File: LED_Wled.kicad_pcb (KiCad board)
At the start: 2 copper layers, 62 x 43 mm, 54 parts, among them J1 SWD_PORT_SKEDD, J2 Barrel_Jack, J3 VIN-Out, J4 MIC_input, J5 LED_signal_chan, J6 +5V Out, Q1 AO4485, Q2 AO4485, Q3 MMBT3904, Q4 AO4485, Q5 AO4485, Q6 MMBT3904, U1 ESP32-WROOM-32, U2 TPS5450DDAR, U3 AMS1117-3.3, U4 SN74HC125DR

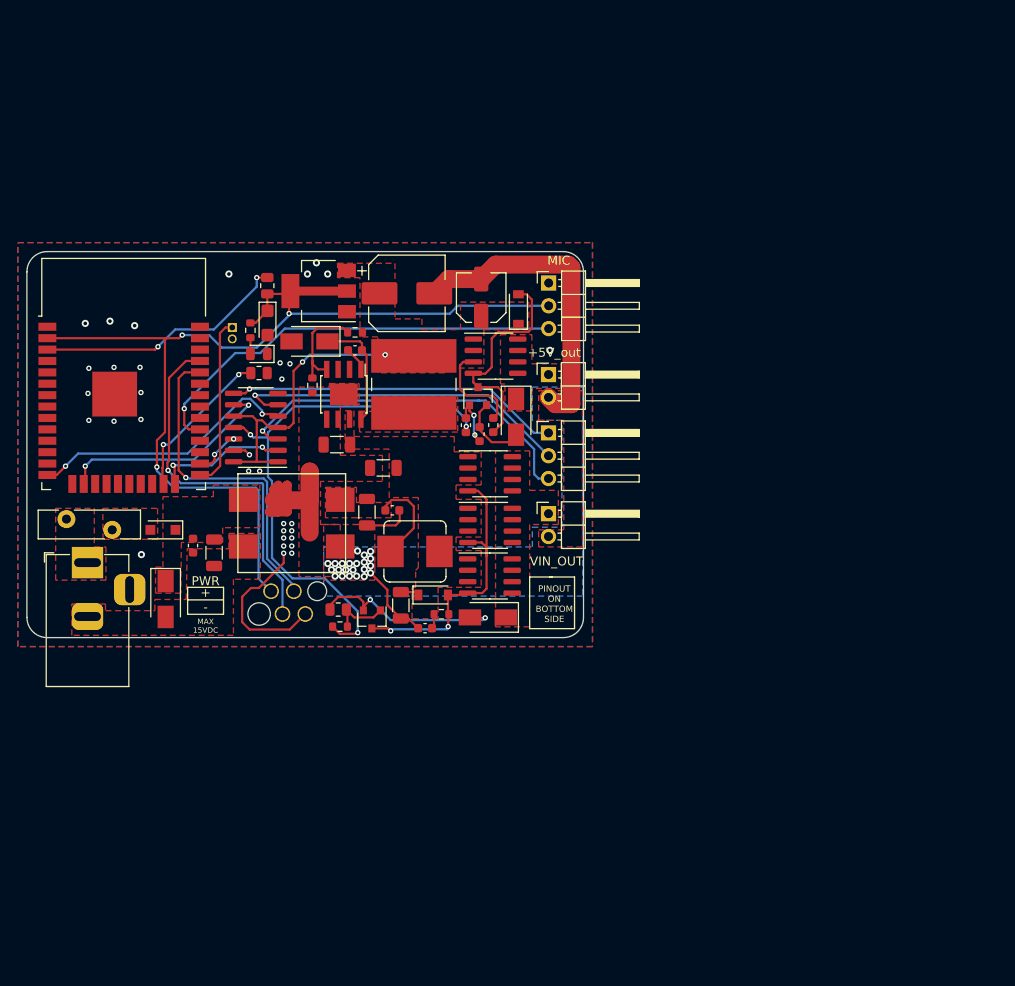
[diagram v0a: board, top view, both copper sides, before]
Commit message: rev2.01
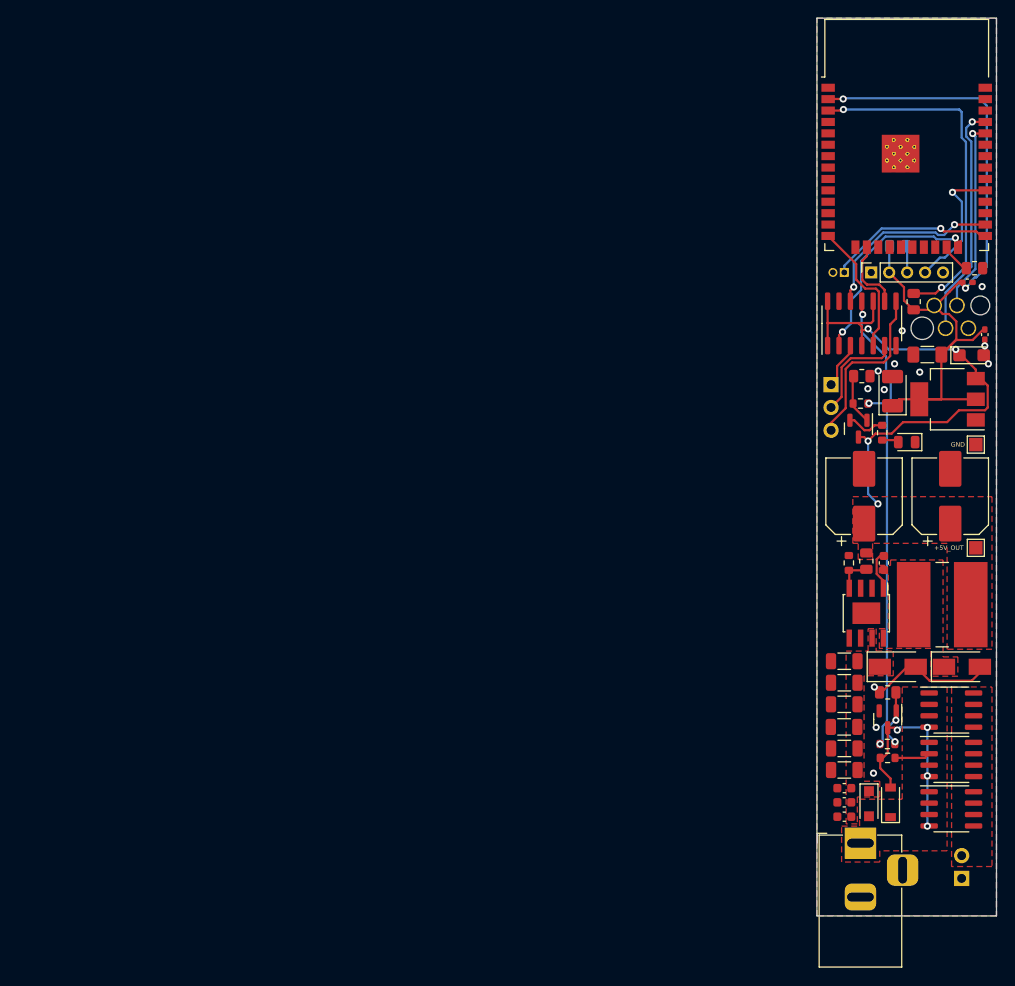
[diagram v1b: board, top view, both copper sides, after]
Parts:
- removed D6, D8: SS34, Diode_SMD:D_SMA
- removed D7: BZT52B15, Diode_SMD:D_SOD-123
- removed F1: Polyfuse, Fuse:Fuse_Bourns_MF-RG650
- removed the G*** at (139.8, 98.5)
- removed L2: 3.3 µH, 6.6 A, Inductor_SMD:L_Bourns_SRP7028A_7.3x6.6mm
- removed L3: ACM1211, userdvc:ACM1211
- removed NT1: Net-Tie_2, NetTie:NetTie-2_SMD_Pad2.0mm
- removed Q6: MMBT3904, Package_TO_SOT_SMD:SOT-23
- added C13: 220 uF 16V, Capacitor_SMD:CP_Elec_8x6.7, F.Cu at (204.8, 103.2)
- added C14: 10uF 16V, Capacitor_Tantalum_SMD:CP_EIA-3216-10_Kemet-I, F.Cu at (207.2, 87.5)
- added C15: 100nF 16V, Capacitor_SMD:C_0402_1005Metric_Pad0.74x0.62mm_HandSolder, F.Cu at (208.7, 85.2)
- added C16: 1uF 25V, Capacitor_SMD:C_0402_1005Metric_Pad0.74x0.62mm_HandSolder, F.Cu at (206.8, 79.4)
- added C17: 100uF 6.3V, Capacitor_SMD:C_1206_3216Metric_Pad1.33x1.80mm_HandSolder, F.Cu at (202.3, 87.5)
- added G***: LOGO, LED_Wled:easyled, B.Cu at (200.0, 60.0)
- added J7: 5V_TP, TestPoint:TestPoint_Pad_1.5x1.5mm, F.Cu at (207.7, 97.5)
- C2: value 150 uF 16V -> 220 uF 16V
- C3: value 22uF 16V -> 22uF/25V; footprint Capacitor_SMD:C_Elec_5x5.4 -> Capacitor_SMD:C_1206_3216Metric
- C4, C5: value 10uF 50V -> 22uF/25V
- C6: value 22uF 10V -> 100uF 6.3V; footprint Capacitor_Tantalum_SMD:CP_EIA-3216-10_Kemet-I -> Capacitor_Tantalum_SMD:CP_EIA-3528-12_Kemet-T_Pad1.50x2.35mm_HandSolder
- J3: value VIN-Out -> LED_VOut; moved to B.Cu
- J4: value MIC_input -> Microphone connector; footprint Connector_PinHeader_2.54mm:PinHeader_1x03_P2.54mm_Horizontal -> Connector_PinSocket_2.00mm:PinSocket_1x05_P2.00mm_Vertical
- J5: moved to B.Cu
- J6: value +5V Out -> Conn_01x01; footprint Connector_PinHeader_2.54mm:PinHeader_1x02_P2.54mm_Horizontal -> TestPoint:TestPoint_Pad_1.5x1.5mm
- L1: value 22uH/5A -> 10uH/6.5A
- Q1: value AO4485 -> MMBT3904; footprint Package_SO:SOIC-8_3.9x4.9mm_P1.27mm -> Package_TO_SOT_SMD:SOT-23
- R11: footprint Resistor_SMD:R_0603_1608Metric -> Resistor_SMD:R_0805_2012Metric
- R2: value 4.7k -> 47ohm
- R4: value 4.7k -> 10k; footprint Resistor_SMD:R_0603_1608Metric -> Resistor_SMD:R_0805_2012Metric
- R8: value 15k -> 0ohm; footprint Resistor_SMD:R_0603_1608Metric -> Resistor_SMD:R_0805_2012Metric; moved to B.Cu
- R9: value 4.7k -> 3.3k
- moved J2 91.6 mm to (194.8, 141.9)
- moved U1 91.2 mm to (200.0, 66.0)
- moved D3 84.4 mm to (195.8, 137.5), turned to -90 degrees
- moved D4 81.9 mm to (199.0, 122.2), turned to 0 degrees
- moved D2 81.2 mm to (206.2, 122.2), turned to 0 degrees
- moved R3 80.5 mm to (207.6, 77.8)
- moved J1 80.4 mm to (205.0, 83.3)
- moved C7 77.4 mm to (193.1, 135.8), turned to 0 degrees
- moved C8 74.3 mm to (193.1, 133.8), turned to 0 degrees
- moved D1 72.8 mm to (200.0, 97.2)
- moved R1 72.0 mm to (200.8, 81.6)
- moved R2 71.3 mm to (197.3, 96.2)
- moved U3 71.1 mm to (204.6, 92.5)
- moved C6 70.0 mm to (198.4, 91.5), turned to 90 degrees
- moved U4 68.5 mm to (195.0, 84.0), turned to 90 degrees
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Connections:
- net Net-(C1-Pad1) renamed /PH
- net Net-(C1-Pad2) renamed /BOOT
- C10 pad 1: GNDPWR -> GND
- C10 pad 2: Net-(C10-Pad2) -> VIN_F+
- C11 pad 1: GNDPWR -> GND
- C11 pad 2: Vin -> VIN_F+
- C12 pad 1: GNDPWR -> GND
- C12 pad 2: Vin -> VIN_F+
- C2 pad 2: GNDPWR -> GND
- C3 pad 1: +5V -> GND
- C3 pad 2: GNDPWR -> VIN_F+
- C4 pad 1: GNDPWR -> GND
- C4 pad 2: Vin -> VIN_F+
- C5 pad 1: GNDPWR -> GND
- C5 pad 2: Vin -> VIN_F+
- C7 pad 1: VBat- -> GND
- C7 pad 2: /PWR_Line -> VIN_F+
- C8 pad 1: VBat- -> GND
- C8 pad 2: /PWR_Line -> VIN_F+
- C9 pad 1: GNDPWR -> GND
- C9 pad 2: Net-(C10-Pad2) -> VIN_F+
- D3 pad 1: /PWR_Line -> VIN_F+
- D3 pad 2: Net-(D3-Pad2) -> VIN
- D4 pad 1: /PWR_Line -> VIN_F+
- D4 pad 2: VBat- -> GND
- D5 pad 1: Vin -> VIN
- J2 pad 1: VBat+ -> VIN
- J2 pad 2: VBat- -> GND
- J2 pad 3: (no net) -> GND
- J3 pad 1: LED_VOUT -> GND
- J3 pad 2: GNDPWR -> LED_VOUT
- J4 pad 3: MIC -> Net-(J4-Pad3)
- J5 pad 1: LED_OUT_HS3 -> LED_OUT_HS1
- J5 pad 3: LED_OUT_HS1 -> LED_OUT_HS3
- J6 pad 1: LED_5VOUT -> +5V
- Q1 pad 1: +5V -> Net-(Q1-Pad1)
- Q1 pad 2: +5V -> Net-(Q1-Pad2)
- Q2 pad 1: Vin -> VIN
- Q2 pad 2: Vin -> VIN
- Q2 pad 3: Vin -> VIN
- Q3 pad 2: Net-(D6-Pad2) -> GND
- Q4 pad 1: Vin -> VIN
- Q4 pad 2: Vin -> VIN
- Q4 pad 3: Vin -> VIN
- Q5 pad 1: Vin -> VIN
- Q5 pad 2: Vin -> VIN
- Q5 pad 3: Vin -> VIN
- R10 pad 2: Net-(D6-Pad2) -> GND
- R11 pad 1: Net-(Q6-Pad1) -> Net-(Q1-Pad1)
- R11 pad 2: Net-(D8-Pad2) -> GND
- R2 pad 2: +3V3 -> Net-(Q1-Pad2)
- R4 pad 1: +5V -> /VSENSE
- R4 pad 2: Net-(D7-Pad2) -> +5V
- R5 pad 1: Net-(Q6-Pad1) -> Net-(Q1-Pad1)
- R6 pad 1: Vin -> VIN
- R8 pad 1: +5V -> Net-(J4-Pad3)
- R8 pad 2: Net-(R8-Pad2) -> +3V3
- R9 pad 1: Net-(R8-Pad2) -> /VSENSE
- R9 pad 2: GNDPWR -> GND
- U2 pad 4: Net-(R8-Pad2) -> /VSENSE
- U2 pad 6: GNDPWR -> GND
- U2 pad 7: Vin -> VIN_F+
- U2 pad 9: GNDPWR -> GND
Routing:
- net GNDPWR: track 58.7 -> 0.00 mm, vias 22 -> 0
- net LED_OUT_HS1: track 40.7 -> 5.24 mm, vias 1 -> 0
- net MIC: track 48.4 -> 15.1 mm
- net +3V3: track 113.8 -> 85.8 mm, vias 3 -> 2
- net LED_OUT_HS2: track 38.5 -> 11.4 mm, vias 1 -> 0
- net Net-(D7-Pad2): track 25.7 -> 0.00 mm
- net Net-(D6-Pad2): track 22.8 -> 0.00 mm, vias 2 -> 0
- net LED_OUT_HS3: track 37.3 -> 19.4 mm, vias 1 -> 0
- net GND: track 31.0 -> 14.0 mm, vias 33 -> 12
- net LED_OUT_LS3: track 24.8 -> 8.06 mm, vias 2 -> 0
- net LED_VOUT_LSWS: track 5.26 -> 21.1 mm
- net RXD: track 36.7 -> 21.5 mm
- net TXD: track 41.2 -> 26.2 mm
- net LED_OUT_LS2: track 30.2 -> 15.5 mm, vias 2 -> 0
- net Net-(R3-Pad1): track 17.5 -> 3.39 mm, vias 2 -> 0
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- added copper zone on F.Cu, net VIN
- added copper zone on F.Cu, net VIN_F+
- removed copper zone on F.Cu, net /PWR_Line
- removed copper zone on B.Cu, net GNDPWR
- removed copper zone on F.Cu, net GNDPWR
- removed copper zone on F.Cu, net LED_5VOUT
- removed copper zone on F.Cu, net Net-(C10-Pad2)
- removed copper zone on F.Cu, net Net-(D3-Pad2)
- removed copper zone on F.Cu, net VBat+
- removed copper zone on F.Cu, net VBat-
- removed copper zone on F.Cu, net Vin
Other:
- board size 62 x 43 mm -> 20 x 100 mm
- board text added: "GAIN TO VCC"
- board text added: "LED1 LED2 LED3"
- board text added: "SIGNAL OUTPUT"
- board text added: "easyLed rev. 2.01 2023-02-01"
- board text removed: "+3V3"
- board text removed: "+5V_out"
- board text removed: "ESled-Controller 2022-11-16 rev2.0"
- board text removed: "LED1"
- board text removed: "LED2"
- board text removed: "LED3"
- board text removed: "MAX 15VDC"
- board text removed: "MIC"
- board text removed: "PINOUT ON BOTTOM SIDE"
- board text removed: "PWR"
- board text removed: "VIN_OUT"
- board text removed: "VOUT"
